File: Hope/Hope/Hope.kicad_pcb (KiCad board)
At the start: 2 copper layers, 18 x 58 mm, 39 parts, among them J1 USB_B_Micro, J2 Conn_01x02, J3 Conn_01x02, J4 Screw_Terminal_01x02, Q1 AO3401A, Q2 AO3401A, U1 W25Q128JVS, U2 RP2040, U3 RT9013-33GB_C19268157, X1 SX1M12.000M10F30TNN

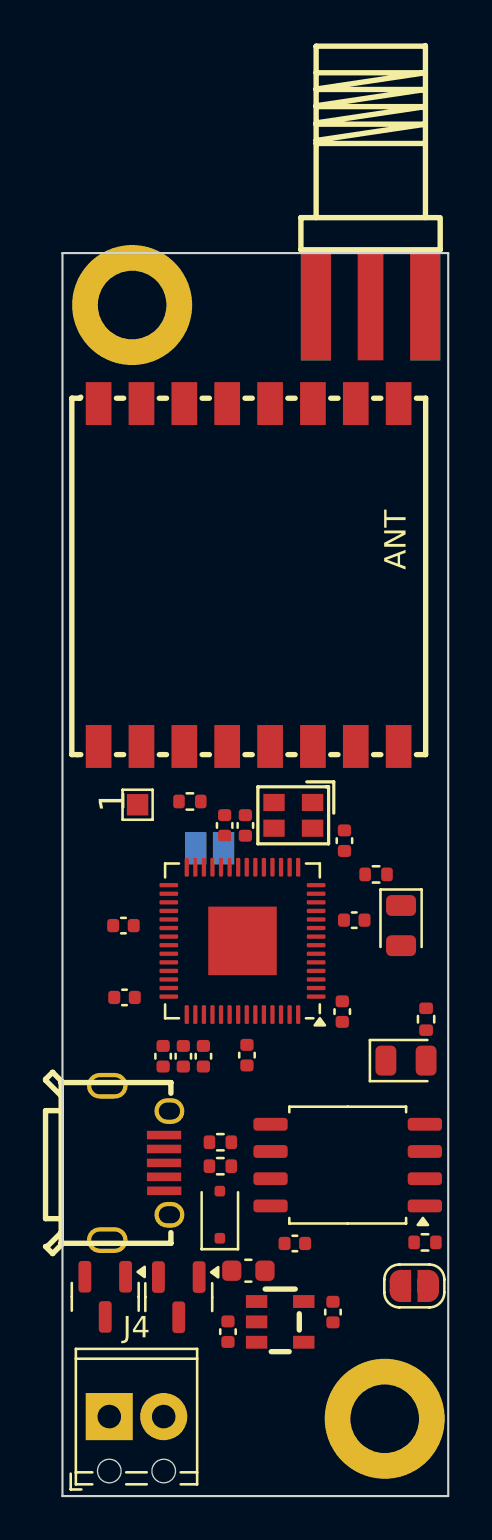
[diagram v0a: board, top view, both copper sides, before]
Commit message: pingpong
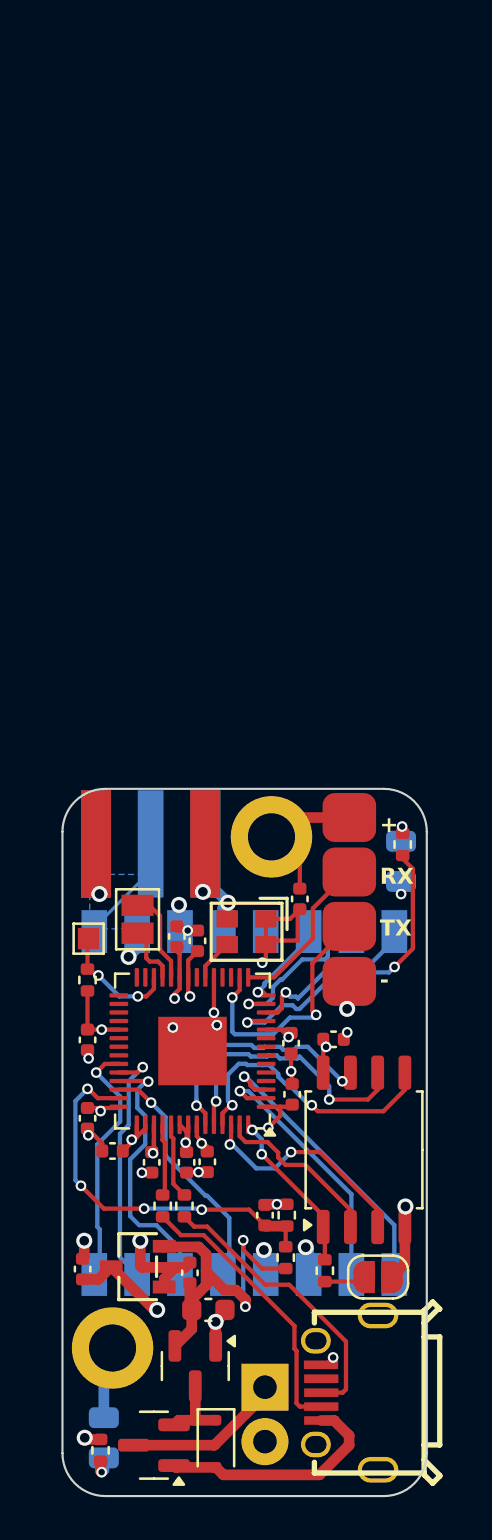
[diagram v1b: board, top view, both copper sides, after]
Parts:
- removed H1, H2: MountingHole_Pad, MountingHole:MountingHole_3.2mm_M3_DIN965_Pad
- added C16: 100n, Capacitor_SMD:C_0402_1005Metric, F.Cu at (201.4, 99.5)
- added H3: MountingHole_Pad, MountingHole:MountingHole_2.2mm_M2_DIN965_Pad, F.Cu at (201.7, 81.8)
- added H4: MountingHole_Pad, MountingHole:MountingHole_2.2mm_M2_DIN965_Pad, F.Cu at (194.3, 105.7)
- added J7: Conn_01x04, .pretty:4 pads 2.54mm spacign, F.Cu at (205.3, 88.5)
- added R8: 30k, Resistor_SMD:R_0402_1005Metric, F.Cu at (202.3, 101.4)
- added R9: 51k, Resistor_SMD:R_0402_1005Metric, F.Cu at (202.4, 99.5)
- AE1, D1, D2, J4, R6: moved to B.Cu
- J2: moved to F.Cu
- U3: value RT9013-33GB_C19268157 -> XC6206P332MR; footprint .pretty:SOT-23-5_L2.9-W1.6-P0.95-LS2.8-BR -> .pretty:SOT-23-3_L2.9-W1.6-P1.90-LS2.8-BR
- moved AE1 27.1 mm to (196.0, 82.1), turned to 180 degrees
- moved R7 25.2 mm to (193.7, 110.4)
- moved R6 24.6 mm to (200.4, 94.2)
- moved D2 22.6 mm to (193.9, 109.9), turned to -90 degrees
- moved J1 14.5 mm to (205.2, 107.7), turned to 90 degrees
- moved C14 11.9 mm to (192.9, 102.0), turned to 90 degrees
- moved D3 10.7 mm to (199.1, 110.1), turned to -90 degrees
- moved C3 9.70 mm to (204.6, 91.3)
- moved R4 9.60 mm to (193.1, 88.5), turned to 90 degrees
- moved J4 7.39 mm to (201.4, 107.5), turned to -90 degrees
- moved Q1 7.29 mm to (196.2, 110.2), turned to 180 degrees
- moved U3 7.13 mm to (195.4, 101.9), turned to 0 degrees
- moved TP1 6.65 mm to (193.1, 86.6)
- moved C7 6.45 mm to (202.6, 91.4), turned to -90 degrees
- moved C11 5.90 mm to (193.1, 94.9), turned to -90 degrees
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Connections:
- U2 pad 12: /MCU/NSS -> /MCU/DIO1
- U2 pad 13: /MCU/SCK -> /MCU/BUSY
- U2 pad 14: /MCU/MOSI -> /MCU/TXCOEN
- U2 pad 15: /MCU/MISO -> /MCU/GPS_TX
- U2 pad 16: unconnected-(U2-GPIO13-Pad16) -> /MCU/GPS_RX
- U2 pad 2: unconnected-(U2-GPIO0-Pad2) -> /MCU/DIO3
- U2 pad 29: /MCU/DIO3 -> unconnected-(U2-GPIO18-Pad29)
- U2 pad 3: unconnected-(U2-GPIO1-Pad3) -> /MCU/DIO2
- U2 pad 30: /MCU/DIO2 -> unconnected-(U2-GPIO19-Pad30)
- U2 pad 31: /MCU/DIO1 -> unconnected-(U2-GPIO20-Pad31)
- U2 pad 32: /MCU/BUSY -> unconnected-(U2-GPIO21-Pad32)
- U2 pad 37: unconnected-(U2-GPIO25-Pad37) -> /MCU/NSS
- U2 pad 38: unconnected-(U2-GPIO26_ADC0-Pad38) -> /MCU/SCK
- U2 pad 39: unconnected-(U2-GPIO27_ADC1-Pad39) -> /MCU/MOSI
- U2 pad 40: unconnected-(U2-GPIO28_ADC2-Pad40) -> /MCU/MISO
- U2 pad 41: unconnected-(U2-GPIO29_ADC3-Pad41) -> /MCU/BATT SENSE 
- U2 pad 5: /MCU/TXCOEN -> unconnected-(U2-GPIO3-Pad5)
- U2 pad 57: unconnected-(U2-GND-Pad57) -> GND
- U3 pad 1: +BATT -> GND
- U3 pad 2: GND -> +BATT
- U3 pad 3: +BATT -> +3V3
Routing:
- net GND: track 0.00 -> 48.6 mm, vias 0 -> 22
- net +3V3: track 0.00 -> 33.7 mm, vias 0 -> 14
- net /MCU/BATT SENSE : track 0.00 -> 17.9 mm, vias 0 -> 4
- net +BATT: track 0.00 -> 16.9 mm, vias 0 -> 2
- net /MCU/LEDINDICATION: track 0.00 -> 14.6 mm, vias 0 -> 2
- net /MCU/DIO2: track 0.00 -> 13.5 mm, vias 0 -> 1
- net /MCU/USB_D+: track 0.00 -> 13.4 mm
- net /MCU/QSPI_SDO: track 0.00 -> 13.3 mm, vias 0 -> 2
- net /MCU/QSPI_SCLK: track 0.00 -> 13.2 mm, vias 0 -> 2
- net /MCU/USB_D-: track 0.00 -> 13.1 mm
- net /MCU/MOSI: track 0.00 -> 12.7 mm, vias 0 -> 1
- net /MCU/DIO3: track 0.00 -> 12.3 mm, vias 0 -> 1
- net /MCU/GPS_RX: track 0.00 -> 11.9 mm, vias 0 -> 2
- net /MCU/QSPI_SD3: track 0.00 -> 11.9 mm, vias 0 -> 2
- net /MCU/NSS: track 0.00 -> 11.7 mm, vias 0 -> 1
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- added copper zone on In1.Cu, net +1V1
- added copper zone on In1.Cu, net +3V3
- added copper zone on B.Cu, net GND
- added copper zone on In2.Cu, net GND
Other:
- board size 18 x 58 mm -> 17 x 33 mm
- copper layers 2 -> 4
- board text added: "+ -"
- board text added: "+ RX TX -"
- board text added: "PWR"
- board text added: "STAT"
